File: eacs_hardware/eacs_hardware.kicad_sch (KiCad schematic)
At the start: 14 parts, among them Q1 S8050, SW1 SW_Push, U1 ESP32-WROOM-32

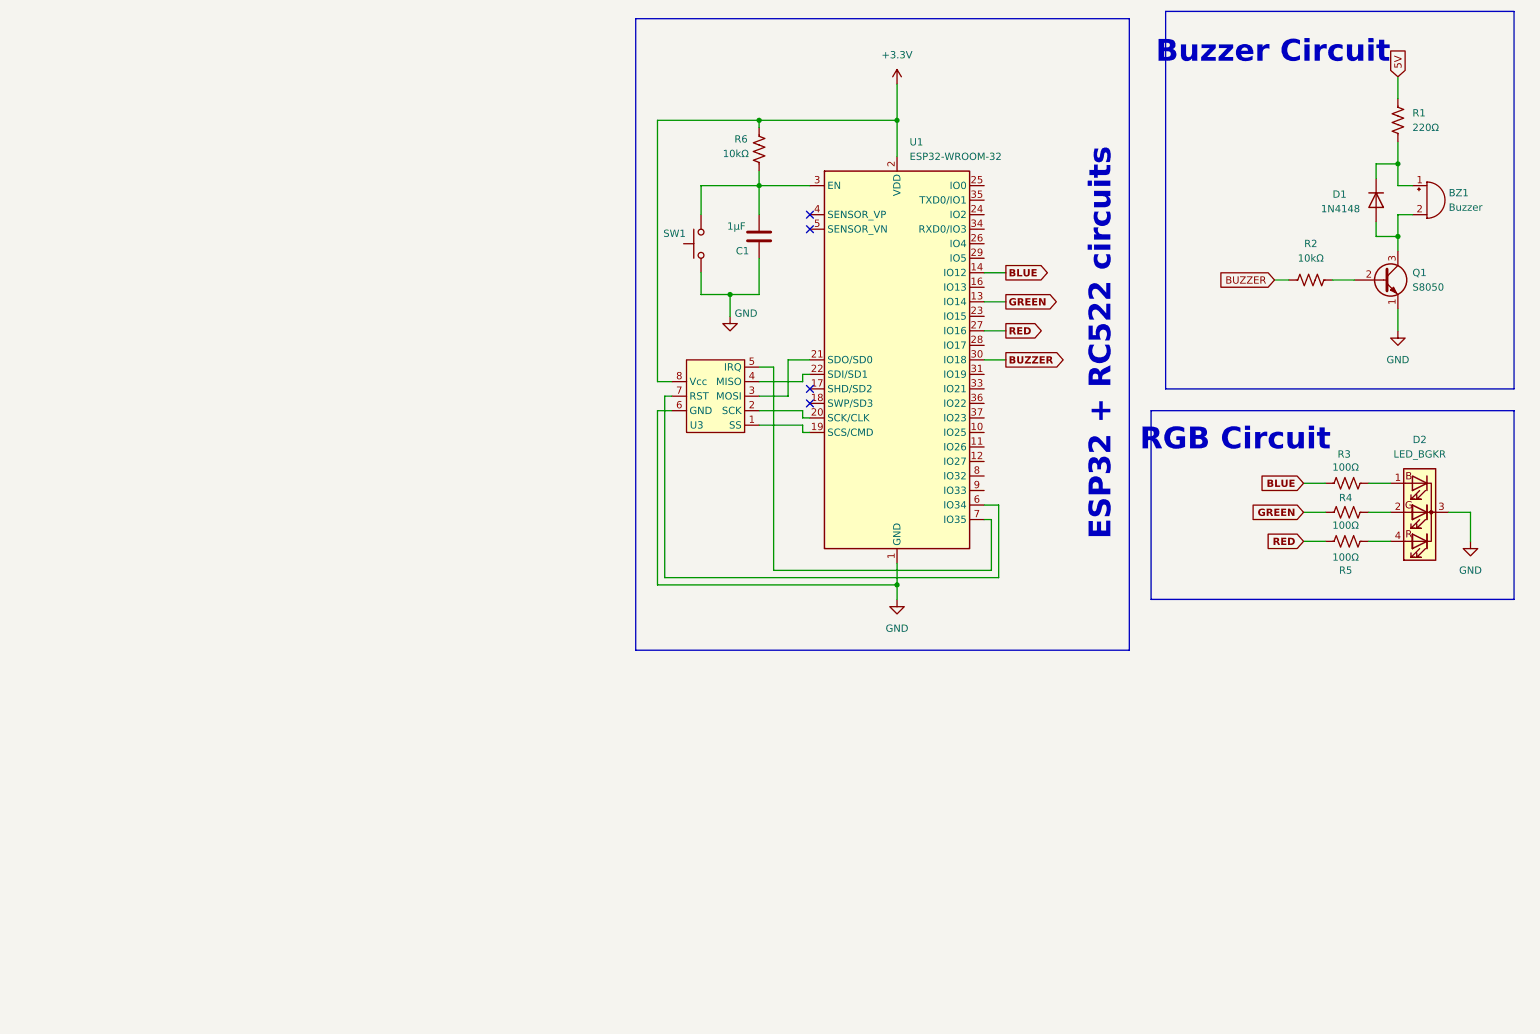
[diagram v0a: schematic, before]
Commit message: Almost done with 5V regulator
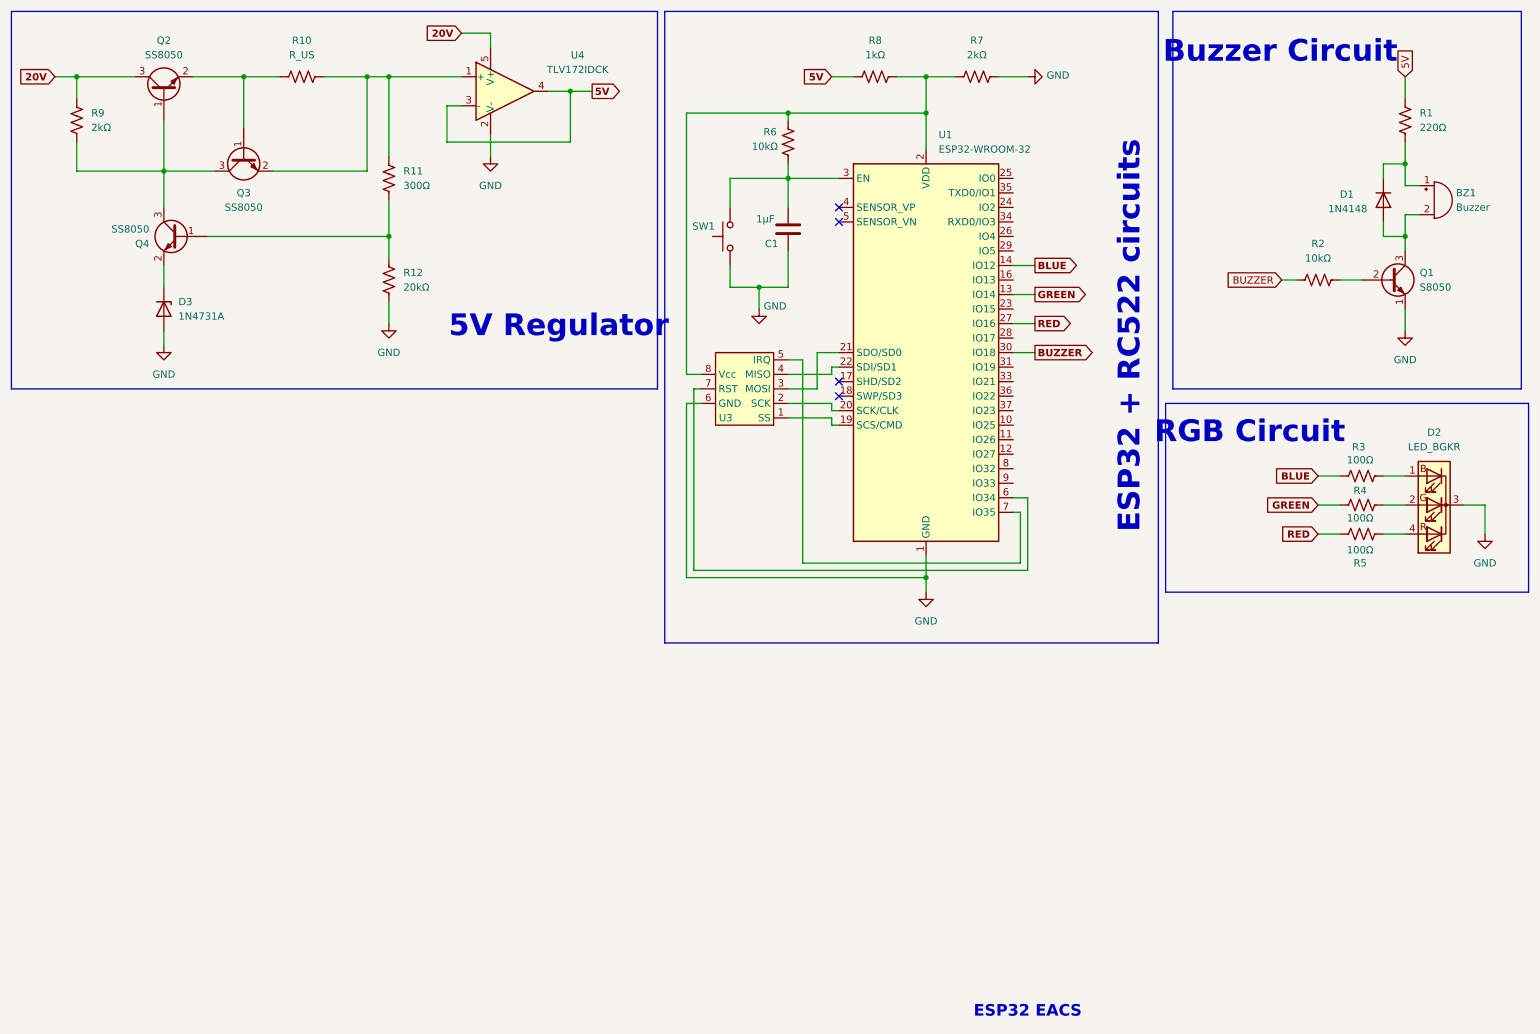
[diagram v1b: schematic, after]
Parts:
- added D3: 1N4731A, Diode_THT:D_DO-41_SOD81_P10.16mm_Horizontal, symbol Diode:1N47xxA
- added Q2, Q3, Q4: SS8050, Package_TO_SOT_SMD:SOT-23, symbol Transistor_BJT:SS8050
- added R10: R_US, symbol Device:R_US
- added R11: 300Ω, symbol Device:R_US
- added R12: 20kΩ, symbol Device:R_US
- added R7, R9: 2kΩ, symbol Device:R_US
- added R8: 1kΩ, symbol Device:R_US
- added U4: TLV172IDCK, Package_TO_SOT_SMD:SOT-353_SC-70-5, symbol Amplifier_Operational:TLV172IDCK
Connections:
- net 5V: now also R8.1, U4.3 (-), U4.4
- net GND: now also D3.2 (A), R12.2, R7.2, U4.2 (V-)
- net +3.3V: no longer names the net of R6.1, U1.2 (VDD), U3.8 (Vcc)
- net +3.3V: now also R7.1, R8.2
- new net: Q2.1 (B), Q3.3 (C), Q4.3 (C), R9.2
- new net: Q2.2 (E), Q3.1 (B), R10.1
- new net: Q4.1 (B), R11.2, R12.1
- new net: D3.1 (K), Q4.2 (E)
- new net: Q3.2 (E), R10.2, R11.1, U4.1 (+)
- new net 20V: Q2.3 (C), R9.1, U4.5 (V+)
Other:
- note added: "5V Regulator"
- note added: "ESP32 EACS"
- moved on the sheet: BZ1, C1, D1, D2, Q1, R1, R2, R3, R4, R5, R6, SW1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
